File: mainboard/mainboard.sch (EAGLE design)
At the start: 48 parts, among them T2 NPN_BC817,215, X1 JST-XH-06-PIN-LONG-PAD

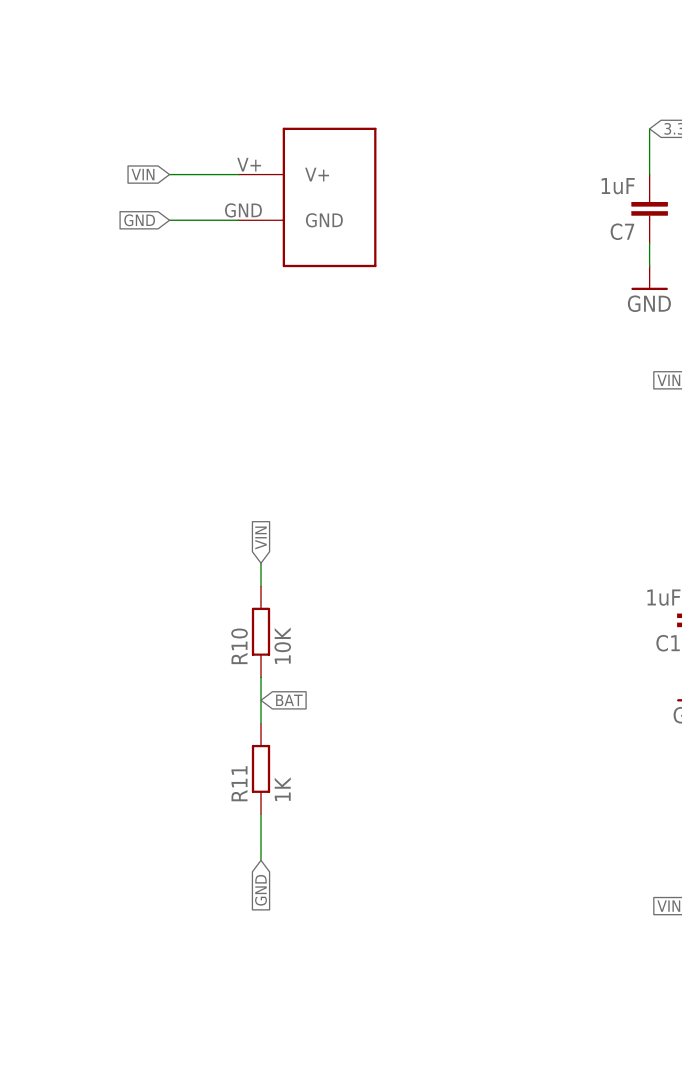
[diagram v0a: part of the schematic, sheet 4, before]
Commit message: mainboard updates
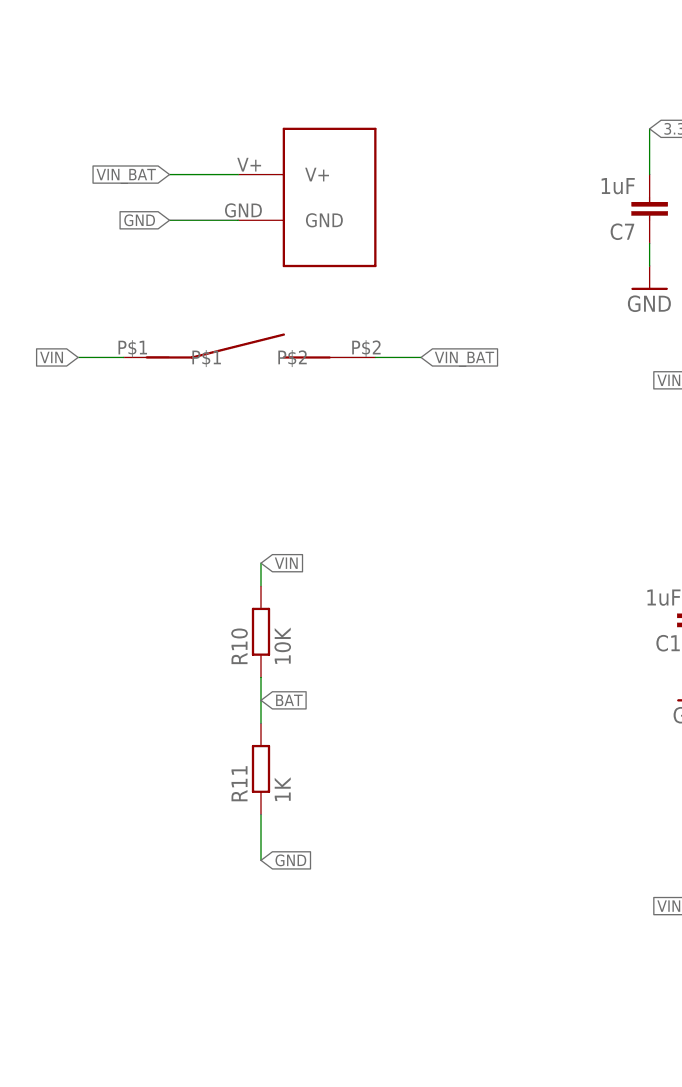
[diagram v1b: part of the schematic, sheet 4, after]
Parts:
- added U$15: SRB22A2FBBNN, rhoban:SRB22A2FBBNN
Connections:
- new net VIN_BAT: U$15.P$2, XT60.V+
- net VIN: now also U$15.P$1; no longer XT60.V+
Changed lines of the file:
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@@
 <attribute name="FARNELL" value="2447553"/>
 </part>
+<part name="U$15" library="rhoban" deviceset="SRB22A2FBBNN" device=""/>
 </parts>
 <sheets>
@@
 <attribute name="FARNELL" x="-45.72" y="-60.96" size="1.778" layer="96" rot="R90" display="off"/>
 </instance>
+<instance part="U$15" gate="G$1" x="-58.42" y="-15.24"/>
 </instances>
 <busses>
@@
 <pinref part="R11" gate="G$1" pin="1"/>
 <wire x1="-45.72" y1="-71.12" x2="-45.72" y2="-66.04" width="0.1524" layer="91"/>
-<label x="-45.72" y="-71.12" size="1.27" layer="95" rot="R270" xref="yes"/>
+<label x="-45.72" y="-71.12" size="1.27" layer="95" xref="yes"/>
 </segment>
 </net>
@@
 </segment>
 <segment>
-<pinref part="XT60" gate="G$1" pin="V+"/>
-<wire x1="-48.26" y1="5.08" x2="-55.88" y2="5.08" width="0.1524" layer="91"/>
-<label x="-55.88" y="5.08" size="1.27" layer="95" rot="R180" xref="yes"/>
-</segment>
-<segment>
 <pinref part="R10" gate="G$1" pin="2"/>
 <wire x1="-45.72" y1="-40.64" x2="-45.72" y2="-38.1" width="0.1524" layer="91"/>
-<label x="-45.72" y="-38.1" size="1.27" layer="95" rot="R90" xref="yes"/>
+<label x="-45.72" y="-38.1" size="1.27" layer="95" xref="yes"/>
+</segment>
+<segment>
+<pinref part="U$15" gate="G$1" pin="P$1"/>
+<wire x1="-60.96" y1="-15.24" x2="-66.04" y2="-15.24" width="0.1524" layer="91"/>
+<label x="-66.04" y="-15.24" size="1.27" layer="95" rot="R180" xref="yes"/>
 </segment>
 </net>
@@
 </segment>
 </net>
+<net name="VIN_BAT" class="2">
+<segment>
+<pinref part="XT60" gate="G$1" pin="V+"/>
+<wire x1="-48.26" y1="5.08" x2="-55.88" y2="5.08" width="0.1524" layer="91"/>
+<label x="-55.88" y="5.08" size="1.27" layer="95" rot="R180" xref="yes"/>
+</segment>
+<segment>
+<pinref part="U$15" gate="G$1" pin="P$2"/>
+<wire x1="-33.02" y1="-15.24" x2="-27.94" y2="-15.24" width="0.1524" layer="91"/>
+<label x="-27.94" y="-15.24" size="1.27" layer="95" xref="yes"/>
+</segment>
+</net>

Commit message: Update mainboard
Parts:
- U$15: FARNELL (none) -> 1383947
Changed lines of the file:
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@@
 <attribute name="FARNELL" value="2447553"/>
 </part>
-<part name="U$15" library="rhoban" deviceset="SRB22A2FBBNN" device=""/>
+<part name="U$15" library="rhoban" deviceset="SRB22A2FBBNN" device="">
+<attribute name="FARNELL" value="1383947"/>
+</part>
 </parts>
 <sheets>
@@
 <attribute name="FARNELL" x="-45.72" y="-60.96" size="1.778" layer="96" rot="R90" display="off"/>
 </instance>
-<instance part="U$15" gate="G$1" x="-58.42" y="-15.24"/>
+<instance part="U$15" gate="G$1" x="-58.42" y="-15.24">
+<attribute name="FARNELL" x="-58.42" y="-15.24" size="1.778" layer="96" display="off"/>
+</instance>
 </instances>
 <busses>
